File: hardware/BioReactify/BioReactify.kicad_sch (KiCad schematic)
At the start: 65 parts, among them IC3 MJ5688-B111-HR1-C, IC4 MJ5688-B111-HR1-C, J10 Conn_01x06_Pin, J16 KF25C-7.62-2P, J17 Conn_01x04_Pin, J18 Conn_01x02, J19 Conn_01x02, J20 Conn_01x02, J21 Conn_01x02, J22 Conn_01x02, J23 Conn_01x02, J9 Conn_01x06_Pin, Q1 IRLZ44N, Q2 IRLZ44N, Q3 IRLZ44N, Q4 IRLZ44N, Q5 IRLZ44N, Q6 IRLZ44N, U1 LD1117S33TR_SOT223, U10 4N25, U11 4N25, U12 4N25, U13 MAX3490xSA, U5 ESP32-DEVKIT-V1, U6 ACS712xLCBTR-030B3, U7 4N25, U8 4N25, U9 4N25

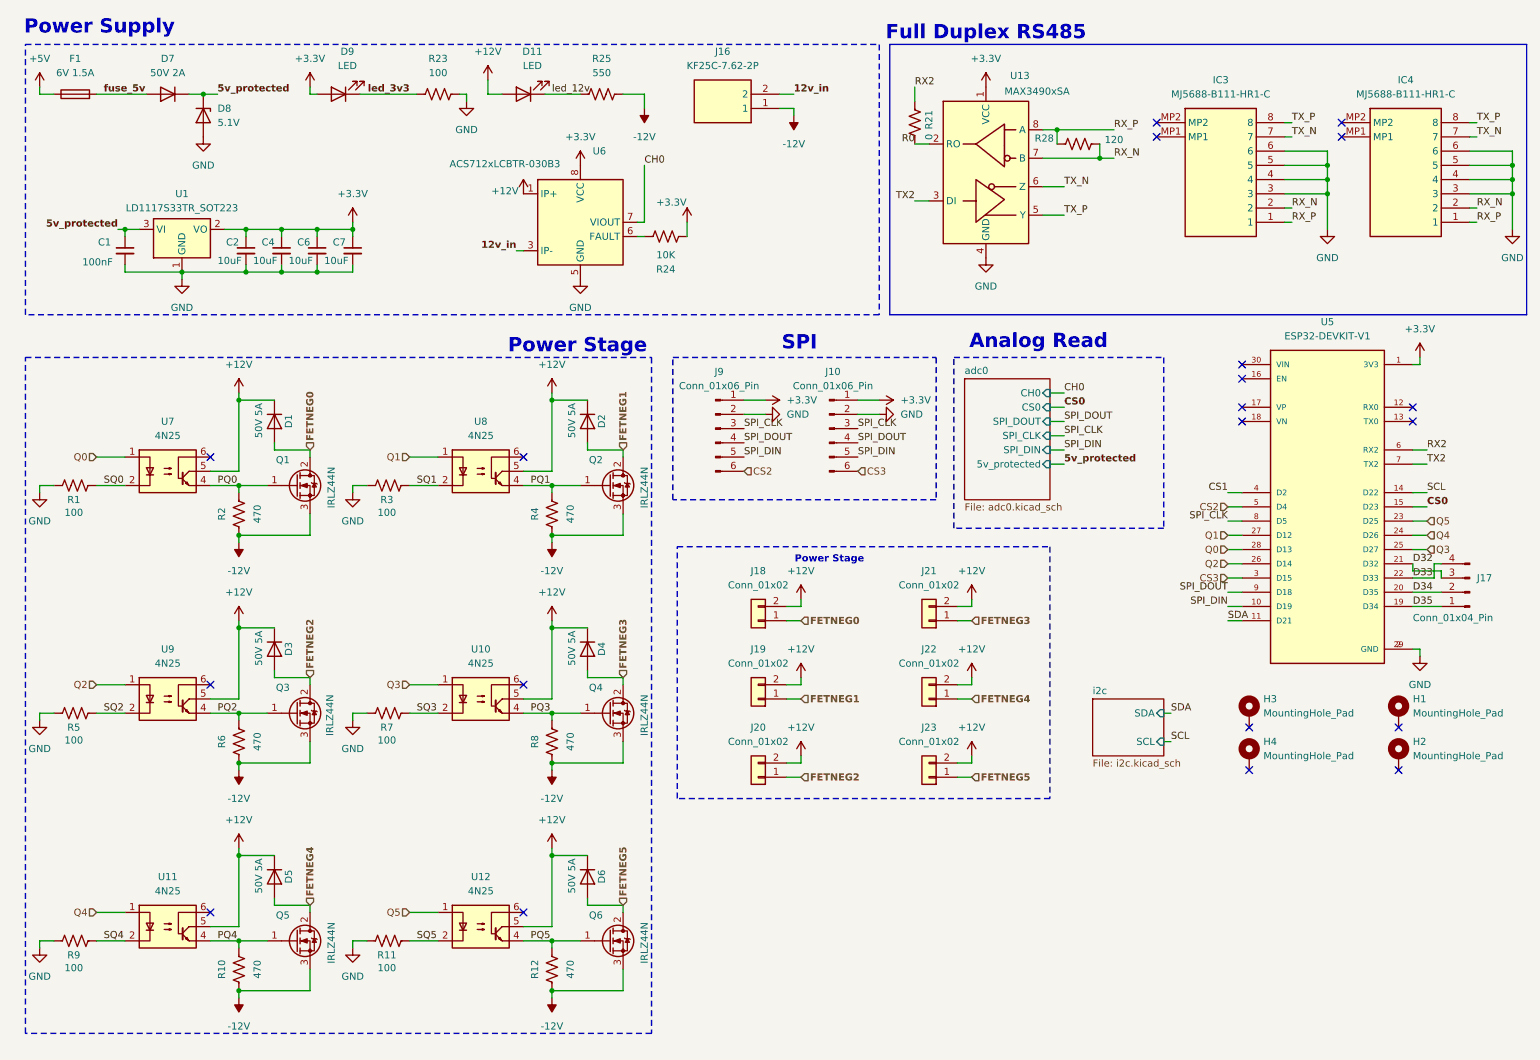
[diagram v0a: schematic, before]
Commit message: PCB complete, biomass sensor PCB complete
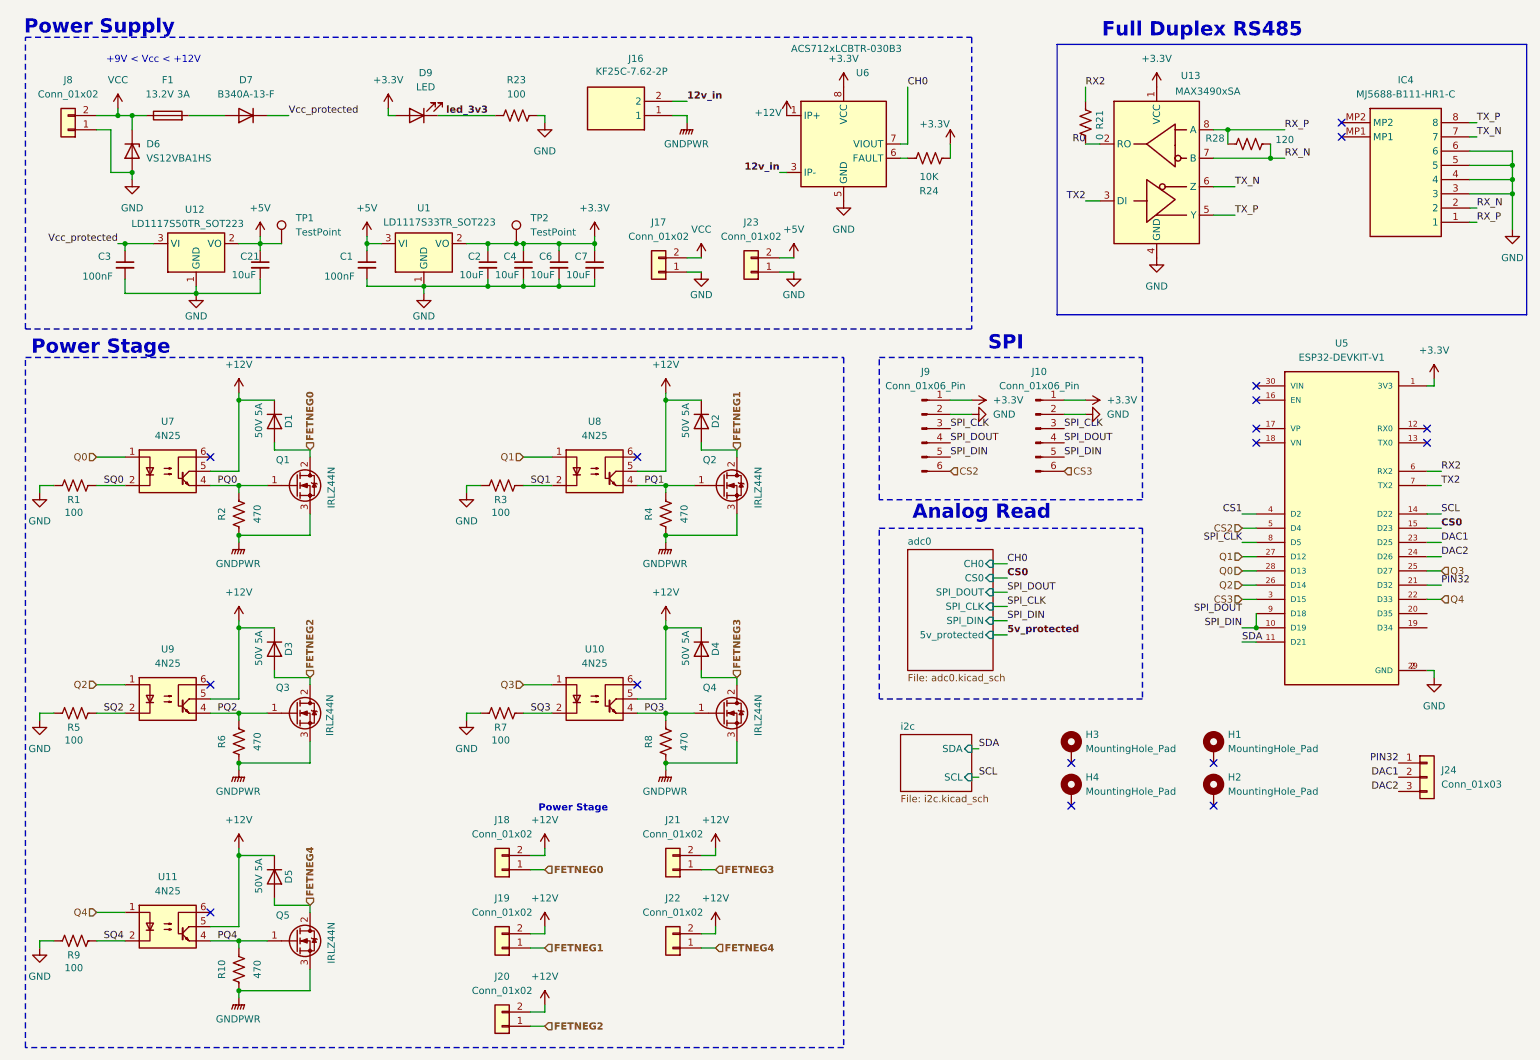
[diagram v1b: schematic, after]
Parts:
- removed D11: LED, LED_SMD:LED_0805_2012Metric, symbol Device:LED
- removed D6: 50V 5A, Diode_SMD:D_SMA, symbol Device:D
- removed D8: 5.1V, Diode_SMD:D_SMB, symbol Device:D_Zener
- removed IC3: MJ5688-B111-HR1-C, SamacSys_Parts:MJ5688B111HR1C, symbol SamacSys_Parts:MJ5688-B111-HR1-C
- removed J17: Conn_01x04_Pin, Connector_PinHeader_2.54mm:PinHeader_1x04_P2.54mm_Vertical, symbol Connector:Conn_01x04_Pin
- removed Q6: IRLZ44N, Package_TO_SOT_THT:TO-220-3_Vertical, symbol Transistor_FET:IRLZ44N
- removed R11: 100, Resistor_SMD:R_0805_2012Metric, symbol Device:R_US
- removed R12: 470, Resistor_SMD:R_0805_2012Metric, symbol Device:R_US
- removed R25: 550, Resistor_SMD:R_0805_2012Metric, symbol Device:R_US
- removed U12: 4N25, Package_DIP:DIP-6_W7.62mm_Socket, symbol Isolator:4N25
- added C21: 10uF, Capacitor_SMD:C_0805_2012Metric, symbol Device:C_Small
- added C3: 100nF, Capacitor_SMD:C_0805_2012Metric, symbol Device:C_Small
- added D6: VS12VBA1HS, Diode_SMD:D_0603_1608Metric_Pad1.05x0.95mm_HandSolder, symbol Device:D_Zener
- added J17, J8: Conn_01x02, Connector_Phoenix_MC:PhoenixContact_MC_1,5_2-G-3.81_1x02_P3.81mm_Horizontal, symbol Connector_Generic:Conn_01x02
- added J24: Conn_01x03, Connector_Phoenix_MC:PhoenixContact_MC_1,5_3-G-3.81_1x03_P3.81mm_Horizontal, symbol Connector_Generic:Conn_01x03
- added TP1, TP2: TestPoint, TestPoint:TestPoint_Pad_1.0x1.0mm, symbol Connector:TestPoint
- added U12: LD1117S50TR_SOT223, Package_TO_SOT_SMD:SOT-223-3_TabPin2, symbol Regulator_Linear:LD1117S50TR_SOT223
- D7: value 50V 2A -> B340A-13-F; footprint Diode_SMD:D_SMB -> Diode_SMD:D_SMA
- F1: value 6V 1.5A -> 13.2V 3A
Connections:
- net D33 is gone; now on net Q4: U5.22 (D33)
- net FETNEG5 is gone; now on net GND: J23.1 (Pin_1)
- net +12V: no longer J23.2 (Pin_2)
- net +3.3V: now also TP2.1
- net +5V: now also C1.1, J23.2 (Pin_2), U1.3 (VI), C21.1, TP1.1, U12.2 (VO); no longer F1.1
- net 5v_protected: no longer C1.1, D7.1 (K), U1.3 (VI)
- net GND: now also C21.2, C3.2, D6.2 (A), J17.1 (Pin_1), J8.1 (Pin_1), U12.1 (GND)
- net Q4: no longer U5.24 (D26)
- net SPI_DIN: now also U5.9 (D18)
- net SPI_DOUT: no longer U5.9 (D18)
- net -12V renamed GNDPWR
- net D32 renamed PIN32
- net PIN32: now also J24.1 (Pin_1)
- net D34: no longer names the net of U5.20 (D35)
- net D35: no longer names the net of U5.19 (D34)
- net Q5 renamed DAC1
- net DAC1: now also J24.2 (Pin_2)
- net fuse_5v: no longer names the net of D7.2 (A), F1.2
- new net DAC2: J24.3 (Pin_3), U5.24 (D26)
- new net VCC: D6.1 (K), F1.1, J17.2 (Pin_2), J8.2 (Pin_2)
- new net Vcc_protected: C3.1, D7.1 (K), U12.3 (VI)
- no-connect marks 20 -> 17
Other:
- note added: "+9V < Vcc < +12V"
- moved on the sheet: C1, C2, C4, C6, C7, D2, D4, D7, D9, F1, H1, H2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
